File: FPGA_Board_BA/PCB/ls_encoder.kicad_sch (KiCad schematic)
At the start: 5 parts, among them U36 SN74LXC2T45Q1

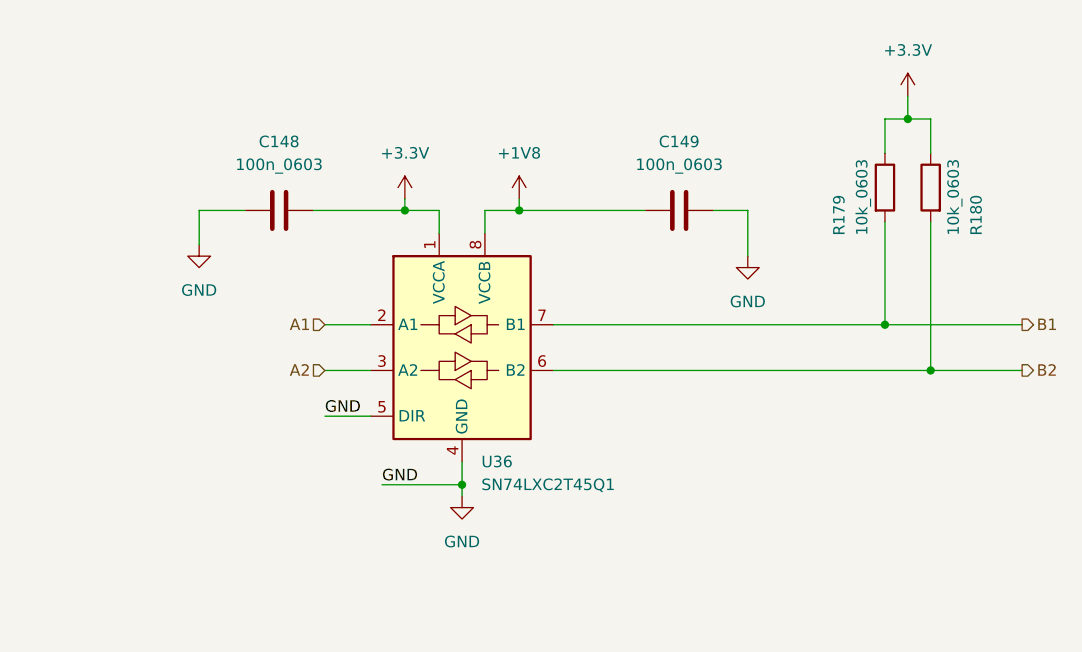
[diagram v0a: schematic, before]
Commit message: 22.11
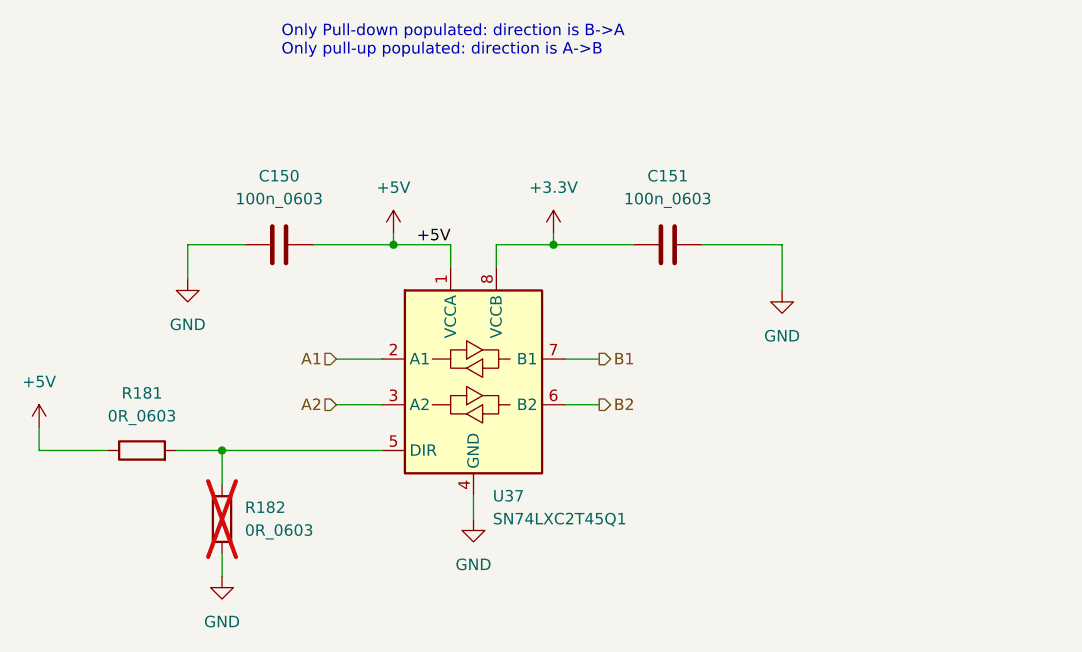
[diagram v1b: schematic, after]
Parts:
- removed C148, C149: 100n_0603, WLIB_Capacitor:C_0603, symbol WLIB_C:100n_0603
- removed R179, R180: 10k_0603, Resistor_SMD:R_0603_1608Metric, symbol WLIB_R:10k_0603
- removed U36: SN74LXC2T45Q1, MYLIB_Misc:SN74LXC2T45QDCURQ1, symbol MYLIB_Misc:SN74LXC2T45Q1
- added C150, C151: 100n_0603, WLIB_Capacitor:C_0603, symbol WLIB_C:100n_0603
- added R181, R182: 0R_0603, Resistor_SMD:R_0603_1608Metric, symbol WLIB_R:0R_0603
- added U37: SN74LXC2T45Q1, MYLIB_Misc:SN74LXC2T45QDCURQ1, symbol MYLIB_Misc:SN74LXC2T45Q1
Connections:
- net +3.3V: now also C151.1, U37.8 (VCCB)
- net A1: now also U37.2 (A1)
- net A2: now also U37.3 (A2)
- net B1: now also U37.7 (B1)
- net B2: now also U37.6 (B2)
- net GND: now also C150.1, C151.2, R182.1, U37.4 (GND)
- new net: R181.2, R182.2, U37.5 (DIR)
- new net +5V: C150.2, R181.1, U37.1 (VCCA)
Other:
- note added: "Only Pull-down populated: direction is B->A Only pull-up populated: direction is A->B"
